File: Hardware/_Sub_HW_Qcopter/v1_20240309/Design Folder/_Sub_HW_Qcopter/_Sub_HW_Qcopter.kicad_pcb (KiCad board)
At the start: 4 copper layers, 49.9 x 49.9 mm, 293 parts, among them J1601 HDR_1X2_VERT, J1701 HDR_1X2_VERT, J1801 HDR_1X2_VERT, J1901 HDR_1X2_VERT, J2101 FPC_24_R/A-BOTT, J2201 HDR_1X2_5A_THD-RA, J2202 HDR_1X2_VERT_1.25MM, J2203 HDR_1X2_VERT_1.25MM, J2204 HDR_1X2_VERT_1.25MM, J2205 HDR_1X2_VERT_1.25MM, J2701 HDR_1X4_VERT, J2801 HDR_1X3_THD-1.27MM, J2901 RECEPT_RF_50R, J3201 USB_MICRO B_RA, J3202 HDR_1X2_VERT_1.25MM, J501 HDR_1X2_VERT, J601 HDR_1X4_VERT, J701 HDR_1X3_THD-1.27MM, U1001 PI4IOE5V9554ZHEX, U1101 PI4IOE5V9554ZHEX, U1201 PI4IOE5V9554ZHEX, U1301 ICM-20948, U1401 BME280, U2001 W25Q64JVSSIQ, U2301 SN74LVC1G18DCKR, U2302 DRV8837CDSGR, U2401 SN74LVC1G18DCKR, U2402 DRV8837CDSGR, U2501 SN74LVC1G18DCKR, U2502 DRV8837CDSGR, U2601 SN74LVC1G18DCKR, U2602 DRV8837CDSGR, U2701 SN74LVC1G17DCKR, U2702 NX3L1T3157GMZ, U2703 STM32WLE5CCU7, U2901 NX3L1T3157GMZ, U2902 BGS13SN8E6327XTSA1, U3101 ATWILC1000B-MU-Y, U3201 MCP73811T-420I/OT, U3301 TPS613222ADBVR, U3401 TLV74033PDBVR, U3501 TLV74033PDBVR, U3601 TLV74033PDBVR, U3701 TLV74033PDBVR, U501 TLV70313DBVR, U502 TLV70328DBVR, U601 SN74LVC1G17DCKR, U602 STM32U575VIT6Q, U801 MCP6006T-E/OT, X2701 32MHz_10pF_10ppm, X3101 26MHz_10ppm_12pF, X601 16MHz_12pF_10ppm

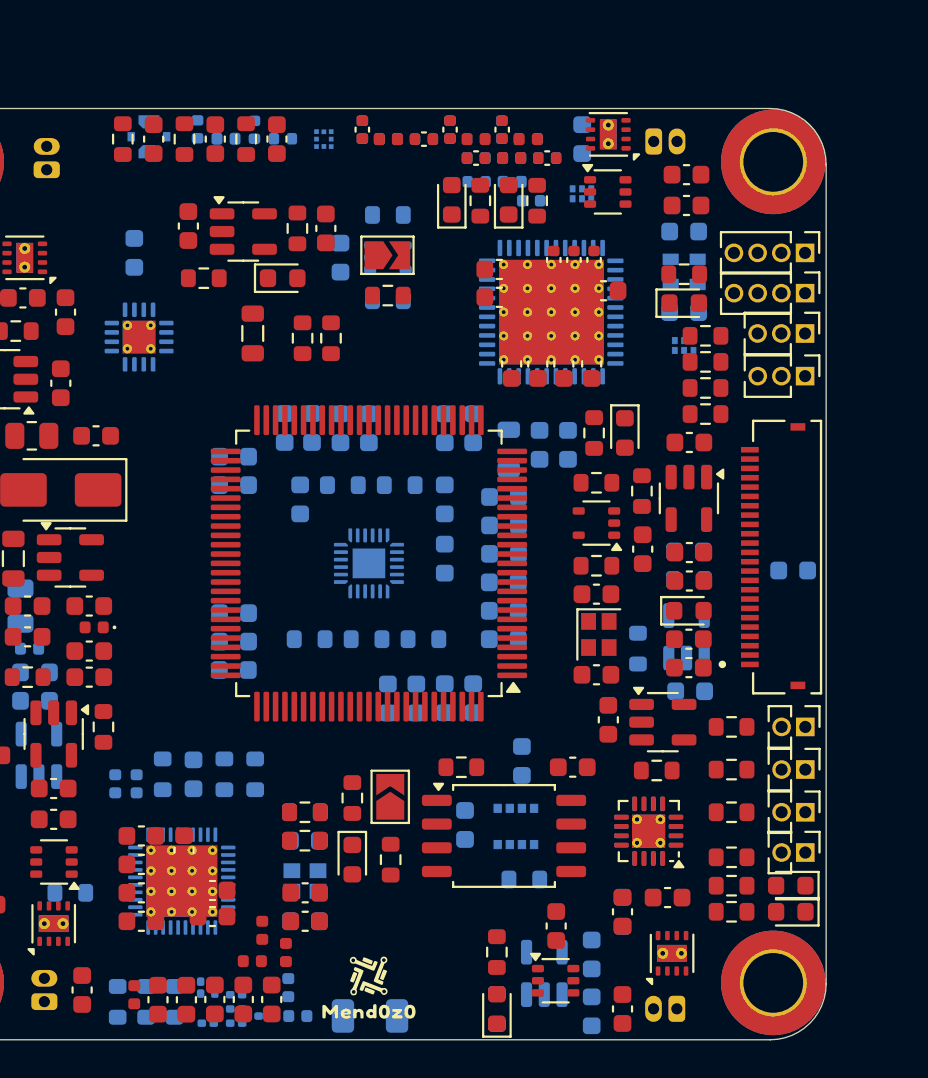
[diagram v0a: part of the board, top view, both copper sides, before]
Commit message: Update _Sub_HW_Qcopter.kicad_pcb
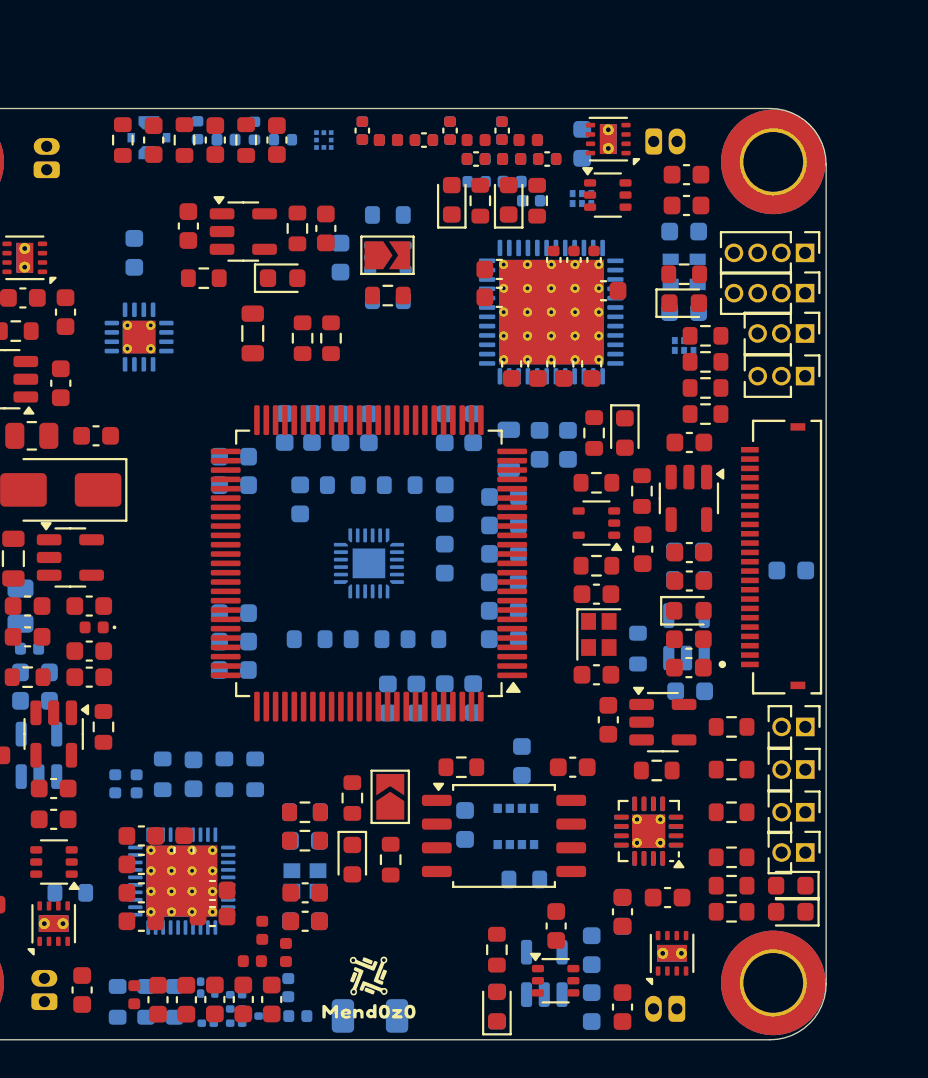
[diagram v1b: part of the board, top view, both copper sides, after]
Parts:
- moved U2502 0.25 mm to (190.6, 205.7)
- moved C2502 0.25 mm to (189.2, 206.0)
- moved U2901 0.25 mm to (189.2, 208.9)
- moved C3701 0.23 mm to (189.7, 252.2)
- moved C3702 0.23 mm to (189.7, 249.2)
- moved U2501 0.17 mm to (190.6, 208.7)
- moved LED3701 0.13 mm to (184.7, 252.2)
- moved R3701 0.13 mm to (184.7, 252.2)
- moved R3702 0.13 mm to (184.7, 249.2)
- moved C2101 0.10 mm to (200.4, 228.9)
- moved C2403 0.10 mm to (191.4, 252.2)
- moved C2904 0.05 mm to (187.4, 206.8)
- moved C2905 0.05 mm to (187.4, 206.8)
- moved C2908 0.05 mm to (184.9, 205.3)
- moved C2909 0.05 mm to (184.9, 205.3)
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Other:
- copper layers 4 -> 6
